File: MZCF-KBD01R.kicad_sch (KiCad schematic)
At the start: 114 parts, among them CN2 XH-4AW_C2908613, SW1 SW_Push, SW10 SW_Push, SW11 SW_Push, SW12 SW_Push, SW13 SW_Push, SW14 SW_Push, SW15 SW_Push, SW16 SW_Push, SW17 SW_Push, SW18 SW_Push, SW19 SW_Push, SW2 SW_Push, SW20 SW_Push, SW21 SW_Push, SW22 SW_Push, SW23 SW_Push, SW24 SW_Push, SW25 SW_Push, SW26 SW_Push, SW27 SW_Push, SW28 SW_Push, SW29 SW_Push, SW3 SW_Push, SW30 SW_Push, SW31 SW_Push, SW32 SW_Push, SW33 SW_Push, SW34 SW_Push, SW35 SW_Push, SW36 SW_Push, SW37 SW_Push, SW38 SW_Push, SW39 SW_Push, SW4 SW_Push, SW40 SW_Push, SW41 SW_Push, SW42 SW_Push, SW43 SW_Push, SW44 SW_Push, SW45 SW_Push, SW46 SW_Push, SW47 SW_Push, SW48 SW_Push, SW49 SW_Push, SW5 SW_Push, SW50 SW_Push, SW51 SW_Push, SW52 SW_Push, SW53 SW_Push, SW54 SW_Push, SW55 SW_Push, SW56 SW_Push, SW6 SW_Push, SW7 SW_Push, SW8 SW_Push, SW9 SW_Push, U1 RP2040-ZERO

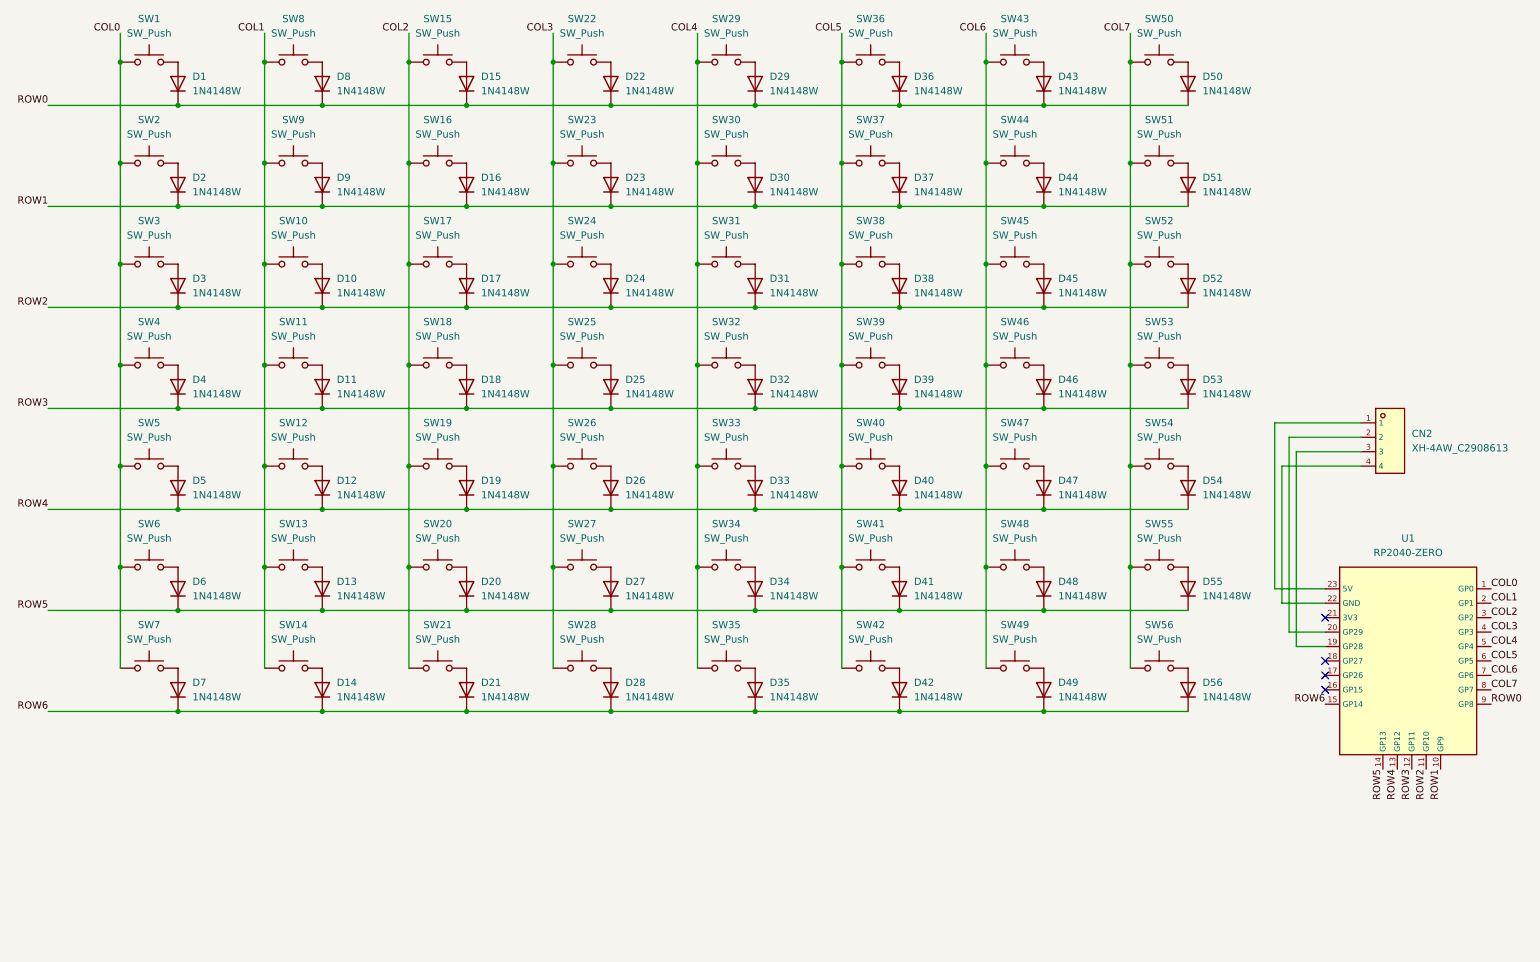
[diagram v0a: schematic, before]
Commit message: feat: new left keyboard
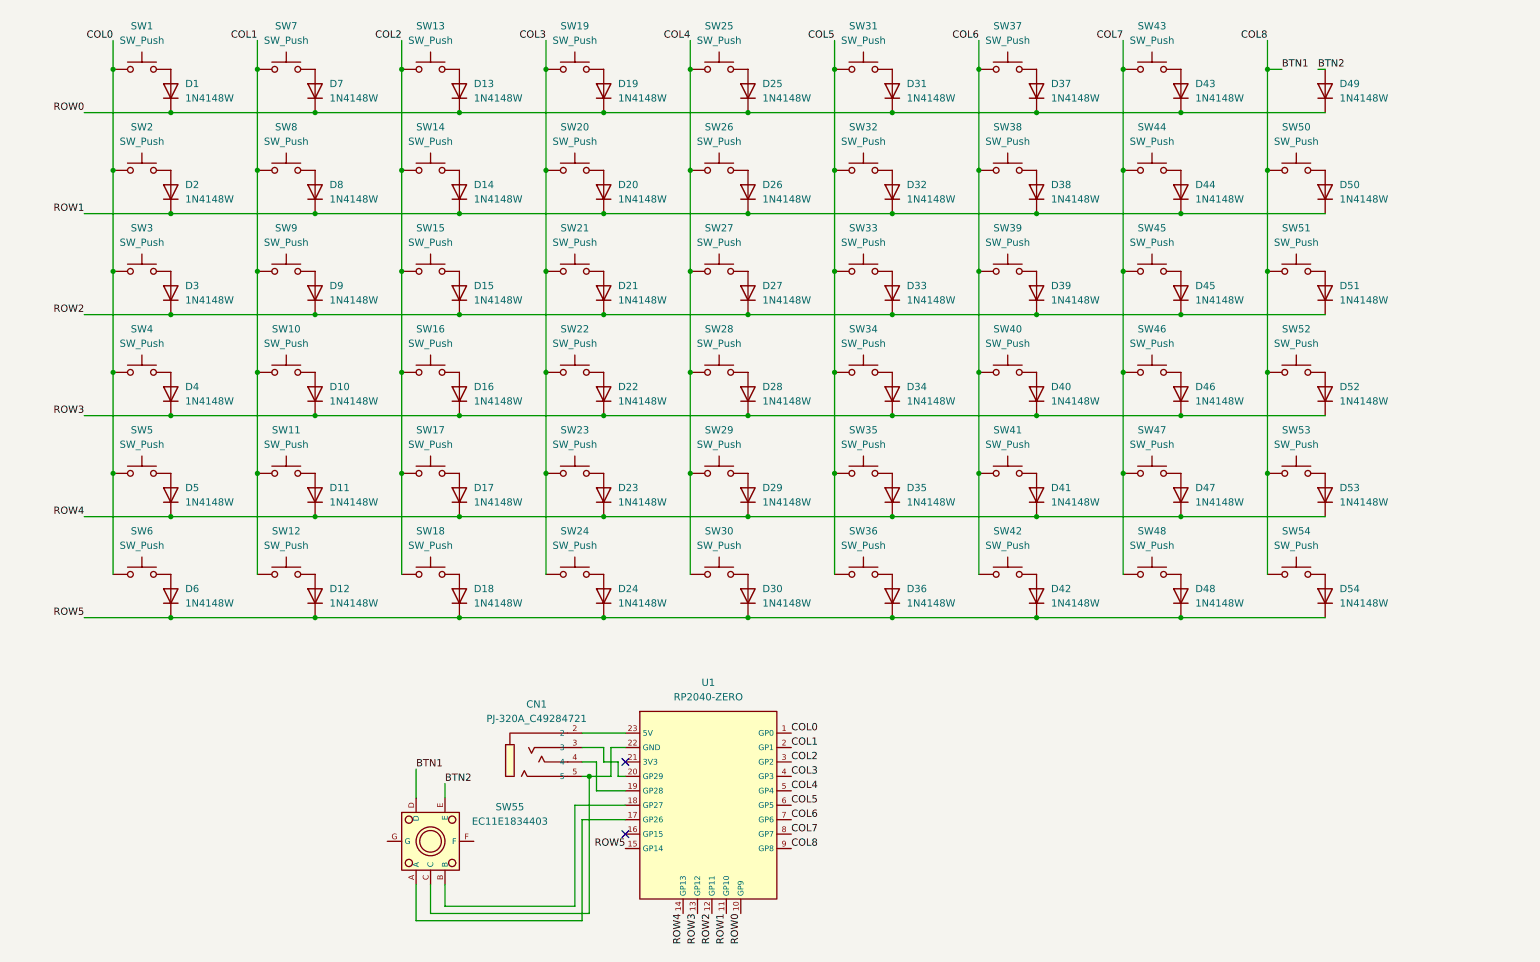
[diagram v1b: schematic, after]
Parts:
- removed CN2: XH-4AW_C2908613, lcsc_footprints:C2908613_CONN-TH_XH-4AW, symbol lcsc_imported:XH-4AW_C2908613
- removed D55, D56: 1N4148W, symbol Diode:1N4148W
- removed SW49, SW55, SW56: SW_Push, symbol Switch:SW_Push
- added CN1: PJ-320A_C49284721, lcsc_footprints:C49284721_AUDIO-TH_PJ-320A_C49284721, symbol lcsc_imported:PJ-320A_C49284721
- added SW55: EC11E1834403, lcsc_footprints:C361165_SW-TH_EC11E1820402, symbol lcsc_imported:EC11E1834403
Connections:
- net COL0: no longer SW7.1
- net COL1: now also SW7.1; no longer SW13.1, SW14.1
- net COL2: now also SW13.1, SW14.1; no longer SW19.1, SW20.1, SW21.1
- net COL3: now also SW19.1, SW20.1, SW21.1; no longer SW25.1, SW26.1, SW27.1, SW28.1
- net COL4: now also SW25.1, SW26.1, SW27.1, SW28.1; no longer SW31.1, SW32.1, SW33.1, SW34.1, SW35.1
- net COL5: now also SW31.1, SW32.1, SW33.1, SW34.1, SW35.1; no longer SW37.1, SW38.1, SW39.1, SW40.1, SW41.1, SW42.1
- net COL6: now also SW37.1, SW38.1, SW39.1, SW40.1, SW41.1, SW42.1; no longer SW43.1, SW44.1, SW45.1, SW46.1, SW47.1, SW48.1
- net COL7: now also SW43.1, SW44.1, SW45.1, SW46.1, SW47.1, SW48.1; no longer SW50.1, SW51.1, SW52.1, SW53.1, SW54.1
- net ROW0: now also D13.1 (K), D19.1 (K), D25.1 (K), D31.1 (K), D37.1 (K), D49.1 (K), D7.1 (K), U1.10 (GP9); no longer D15.1 (K), D22.1 (K), D29.1 (K), D36.1 (K), D50.1 (K), D8.1 (K), U1.9 (GP8)
- net ROW1: now also D14.1 (K), D20.1 (K), D26.1 (K), D32.1 (K), D38.1 (K), D50.1 (K), D8.1 (K), U1.11 (GP10); no longer D16.1 (K), D23.1 (K), D30.1 (K), D37.1 (K), D51.1 (K), D9.1 (K), U1.10 (GP9)
- net ROW2: now also D15.1 (K), D21.1 (K), D27.1 (K), D33.1 (K), D39.1 (K), D51.1 (K), D9.1 (K), U1.12 (GP11); no longer D10.1 (K), D17.1 (K), D24.1 (K), D31.1 (K), D38.1 (K), D52.1 (K), U1.11 (GP10)
- net ROW3: now also D10.1 (K), D16.1 (K), D22.1 (K), D28.1 (K), D34.1 (K), D40.1 (K), D52.1 (K), U1.13 (GP12); no longer D11.1 (K), D18.1 (K), D25.1 (K), D32.1 (K), D39.1 (K), D53.1 (K), U1.12 (GP11)
- net ROW4: now also D11.1 (K), D17.1 (K), D23.1 (K), D29.1 (K), D35.1 (K), D41.1 (K), D53.1 (K), U1.14 (GP13); no longer D12.1 (K), D19.1 (K), D26.1 (K), D33.1 (K), D40.1 (K), D54.1 (K), U1.13 (GP12)
- net ROW5: now also D12.1 (K), D18.1 (K), D24.1 (K), D30.1 (K), D36.1 (K), D42.1 (K), D54.1 (K), U1.15 (GP14); no longer D13.1 (K), D20.1 (K), D27.1 (K), D34.1 (K), D41.1 (K), U1.14 (GP13)
- net at U1.17 (GP26): now also SW55.A
- net at U1.18 (GP27): now also SW55.B
- net at U1.19 (GP28): now also CN1.4
- net at U1.20 (GP29): now also CN1.3
- net at U1.22 (GND): now also CN1.5, SW55.C
- net at U1.23 (5V): now also CN1.2
- net BTN2: now reaches D49.2 (A)
- net BTN2: now also SW55.E
- removed net ROW6: D14.1 (K), D21.1 (K), D28.1 (K), D35.1 (K), D42.1 (K), D49.1 (K), D7.1 (K), U1.15 (GP14)
- new net BTN1: SW50.1, SW51.1, SW52.1, SW53.1, SW54.1, SW55.D, U1.9 (GP8)
- no-connect marks 4 -> 2
